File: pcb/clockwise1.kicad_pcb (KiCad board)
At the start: 2 copper layers, 70.7 x 90.7 mm, 21 parts, among them J1 Jack-DC, J2 JIN, J3 Flash, J4 JOUT, J5 Matrix Power, SW1 BOOT, SW2 Source, SW3 RESET, U1 LM1117-3.3, U2 ESP32-WROOM-32

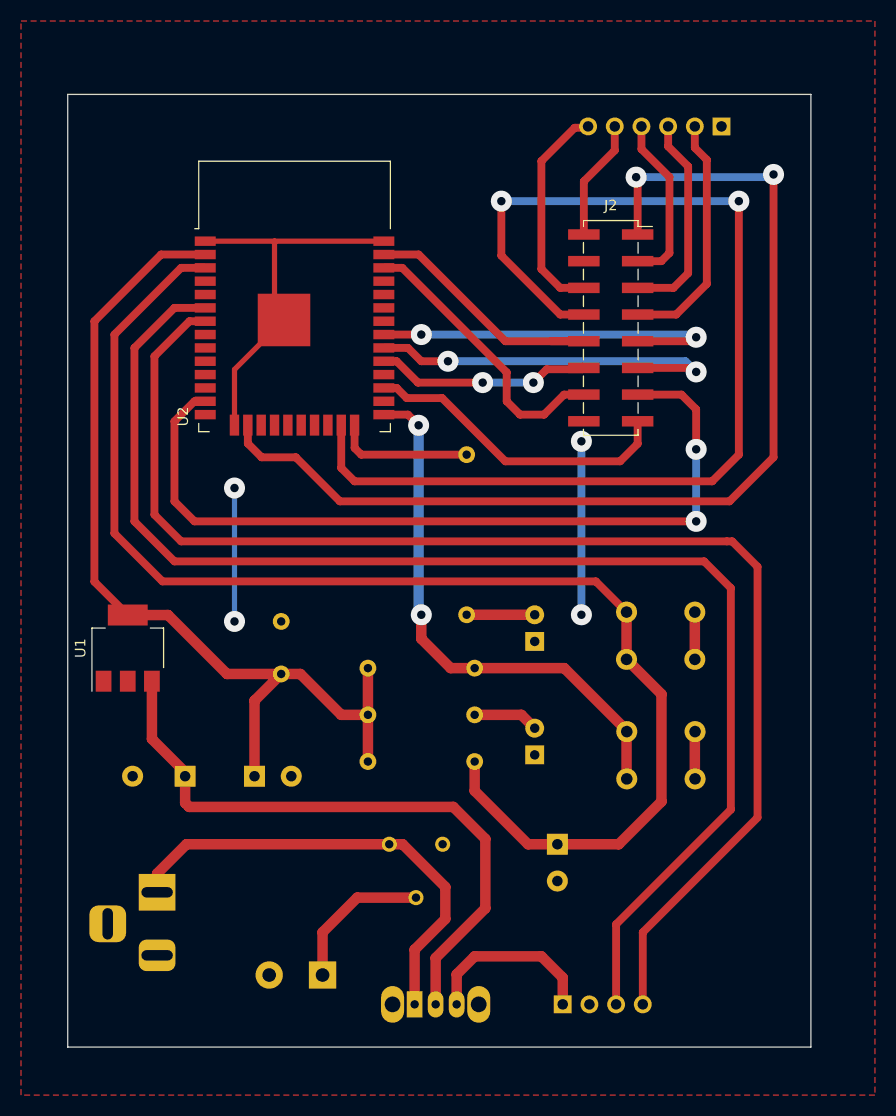
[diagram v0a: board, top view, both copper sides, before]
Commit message: Improvements after first version
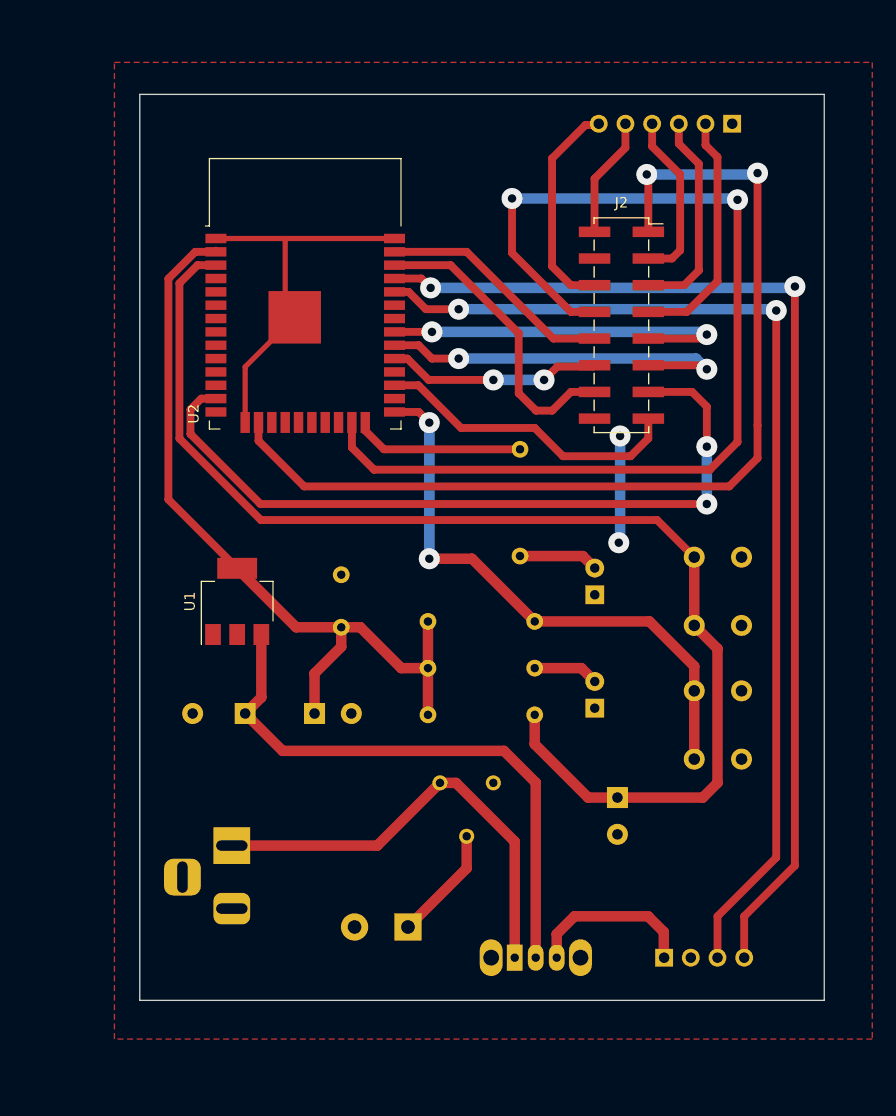
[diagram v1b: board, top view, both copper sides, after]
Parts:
- R3: footprint Resistor_THT:R_Axial_DIN0207_L6.3mm_D2.5mm_P15.24mm_Horizontal -> Resistor_THT:R_Axial_DIN0207_L6.3mm_D2.5mm_P10.16mm_Horizontal
- moved U1 11.3 mm to (115.8, 99.1)
- moved J3 10.6 mm to (156.5, 133.0)
- moved SW1 10.6 mm to (159.3, 107.6), turned to 270 degrees
- moved SW2 10.5 mm to (142.2, 133.0)
- moved J5 9.33 mm to (132.1, 130.0)
- moved J1 8.39 mm to (115.3, 122.3)
- moved C1 8.26 mm to (116.6, 109.7)
- moved C2 8.26 mm to (123.2, 109.7)
- moved RV1 7.58 mm to (140.2, 116.3)
- moved C3 7.24 mm to (125.7, 96.5)
- moved C4 7.24 mm to (152.0, 117.7)
- moved D1 7.24 mm to (149.9, 109.2)
- moved D2 7.24 mm to (149.9, 98.4)
- moved R2 7.24 mm to (144.1, 105.4)
- moved R1 7.24 mm to (134.0, 101.0)
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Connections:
- U2 pad 34: Net-(U2-Pad34) -> RX
- U2 pad 35: Net-(U2-Pad35) -> TX
- U2 pad 6: RX -> Net-(U2-Pad6)
- U2 pad 7: TX -> Net-(U2-Pad7)
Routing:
- net GNDREF: track 75.0 -> 47.1 mm, vias 4 -> 2
- net RX: track 128.4 -> 101.5 mm, vias 0 -> 2
- net TX: track 126.9 -> 104.4 mm, vias 0 -> 2
- net +3V3: track 88.9 -> 76.3 mm
- net EN: track 125.8 -> 117.9 mm
- net R1: track 101.4 -> 95.2 mm
- net CLK: track 78.6 -> 72.5 mm
- net Net-(C1-Pad1): track 60.6 -> 55.2 mm
- net E: track 105.6 -> 101.0 mm
- net Net-(J5-Pad1): track 14.3 -> 11.0 mm
- net IO0: track 51.8 -> 55.0 mm
- net Net-(R3-Pad1): track 13.1 -> 16.2 mm
- net Net-(J1-Pad1): track 44.4 -> 42.8 mm
- net LAT: track 27.2 -> 28.9 mm
- net Net-(D2-Pad2): track 6.48 -> 7.59 mm
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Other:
- board size 70.7 x 90.7 mm -> 65.2 x 86.2 mm
- net class Default: clearance 0.2 -> 0.3
- net class Default2 removed
- net class MCU added: clearance 0.5, trace_width 0.75, via_dia 0.8, via_drill 0.4
- rule trace_clearance: 0.2 -> 0.3
